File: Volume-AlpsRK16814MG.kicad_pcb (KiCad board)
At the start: 2 copper layers, 62.9 x 32.4 mm, 10 parts, among them P1 AB I/O, P2 CD I/O, P3 PWR, P4 CTRL, P5 GND, U1 SN754410

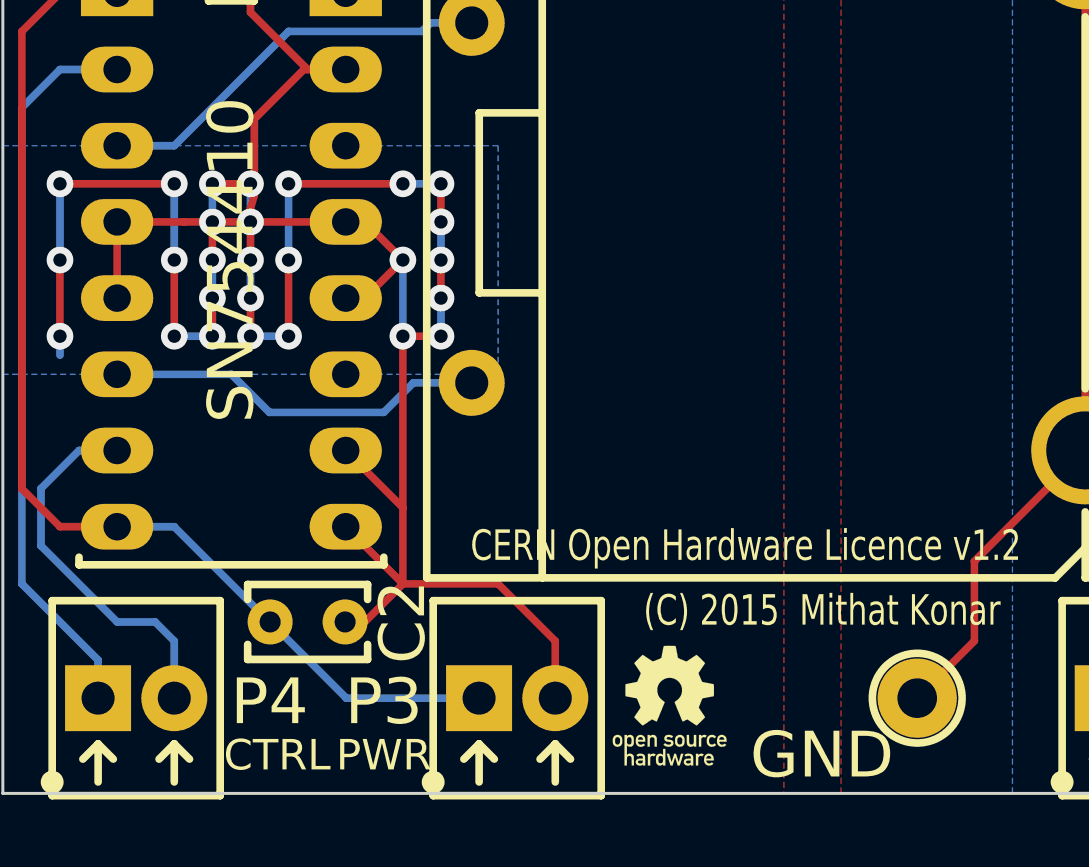
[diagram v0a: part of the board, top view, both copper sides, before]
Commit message: Silk tweaks.
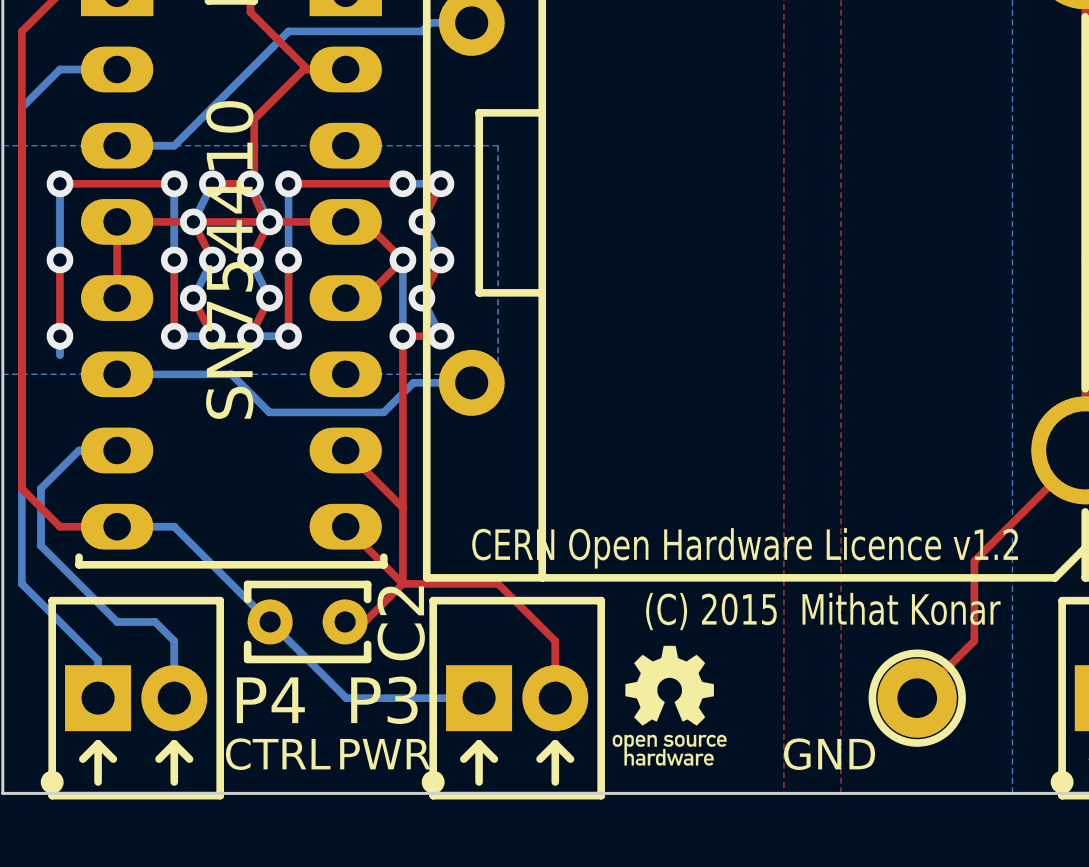
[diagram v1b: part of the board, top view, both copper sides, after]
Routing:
- net DGND: track 100.1 -> 102.0 mm
